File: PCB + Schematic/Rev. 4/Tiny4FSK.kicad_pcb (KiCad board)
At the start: 4 copper layers, 36.3 x 69.2 mm, 84 parts, among them J1 SWD, J2 GPIO, J3 USBC, J4 USB, J5 I2C, J6 Power Ext, J7 SPI, J8 USB Breakout, SW1 RST, SW2 Power Switch, U1 BME280, U2 ATGM336H, U3 SI4063, U4 ATSAMD21G18A-A, U5 1XZA032768AD19, U6 TPS61200DRC, U8 Linear Step-Down

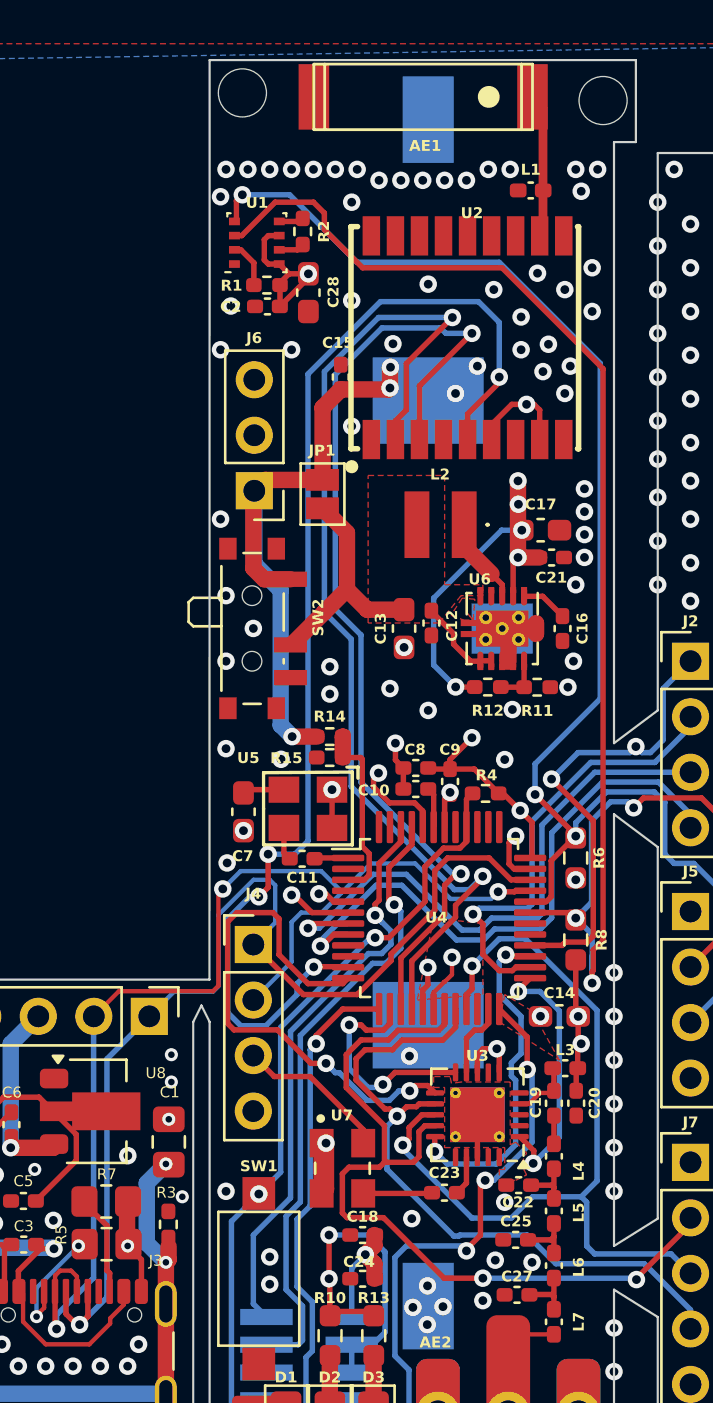
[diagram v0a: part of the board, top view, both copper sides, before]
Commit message: JLCPCB Centroid Fixes
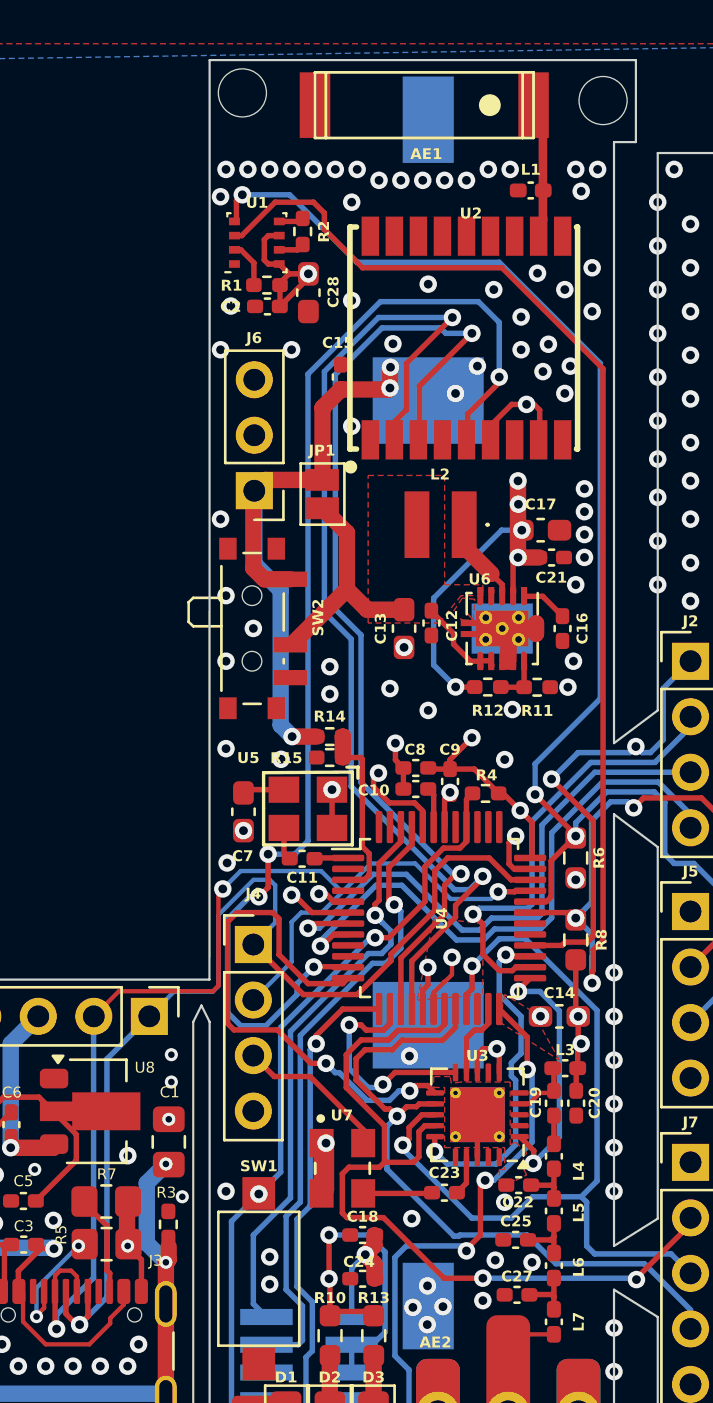
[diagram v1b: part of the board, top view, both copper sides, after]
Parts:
- moved AE1 6.52 mm to (150.0, 45.8), turned to 180 degrees
- moved J3 1.00 mm to (133.9, 102.8)
- moved U2 0.25 mm to (152.0, 56.5)
- turned U4 to -90 degrees
- turned U8 to 180 degrees
